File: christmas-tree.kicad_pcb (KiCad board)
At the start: 2 copper layers, 59 x 53 mm, 11 parts, among them IC1 ATTINY85-P, P1 CONN_2, Q1 PHOTO-TRANSISTOR, SW1 SPST

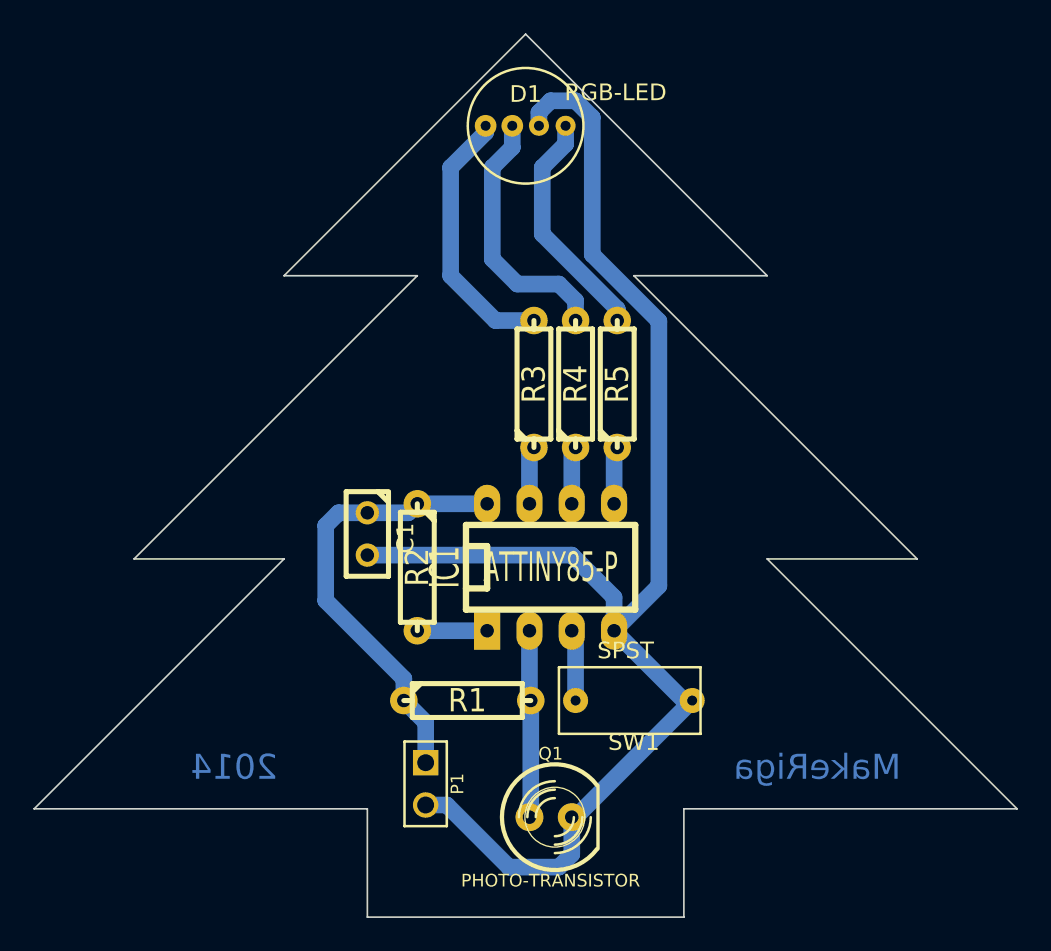
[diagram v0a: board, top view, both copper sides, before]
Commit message: Changes from workstation
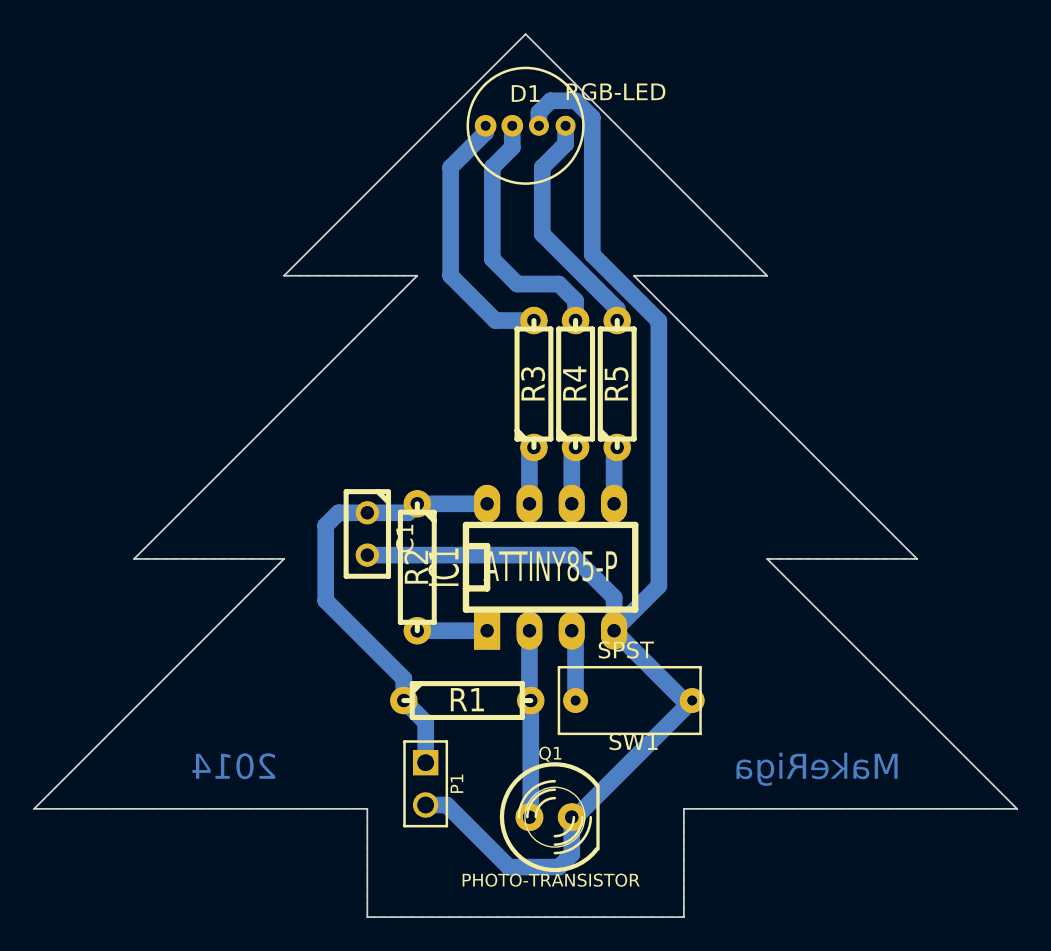
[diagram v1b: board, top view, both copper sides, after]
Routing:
- added copper zone on B.Cu, net (none)
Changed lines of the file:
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@@
     (last_trace_width 1)
     (trace_clearance 0.254)
-    (zone_clearance 0.508)
+    (zone_clearance 1)
     (zone_45_only no)
     (trace_min 0.254)
@@
   (gr_line (start 67 55.5) (end 75 55.5) (angle 90) (layer Edge.Cuts) (width 0.1))
   (gr_line (start 81.5 41) (end 67 55.5) (angle 90) (layer Edge.Cuts) (width 0.1))
-  (segment (start 82.3 46.5) (end 82.3 45.7) (width 1) (layer B.Cu) (net 1) (status 400000))
-  (segment (start 89.5 74.12) (end 86.81 76.81) (width 1) (layer B.Cu) (net 1) (status 800000))
+  (segment (start 82.3 46.5) (end 82.3 45.7) (width 1) (layer B.Cu) (net 1))
+  (segment (start 89.5 74.12) (end 86.81 76.81) (width 1) (layer B.Cu) (net 1))
   (segment (start 89.5 58.226574) (end 89.5 74.12) (width 1) (layer B.Cu) (net 1))
   (segment (start 85.5 54.226574) (end 89.5 58.226574) (width 1) (layer B.Cu) (net 1))
@@
   (segment (start 91.5 81) (end 91 81) (width 1) (layer B.Cu) (net 1))
   (segment (start 91 81) (end 86.81 76.81) (width 1) (layer B.Cu) (net 1))
-  (segment (start 79.1 46.5) (end 79.1 46.9) (width 1) (layer B.Cu) (net 2) (status C00000))
-  (segment (start 79.69 58.19) (end 82 58.19) (width 1) (layer B.Cu) (net 2) (status 800000))
+  (segment (start 79.1 46.5) (end 79.1 46.9) (width 1) (layer B.Cu) (net 2))
+  (segment (start 79.69 58.19) (end 82 58.19) (width 1) (layer B.Cu) (net 2))
   (segment (start 77 55.5) (end 79.69 58.19) (width 1) (layer B.Cu) (net 2))
   (segment (start 77 49) (end 77 55.5) (width 1) (layer B.Cu) (net 2))
-  (segment (start 79.1 46.9) (end 77 49) (width 1) (layer B.Cu) (net 2) (status 400000))
+  (segment (start 79.1 46.9) (end 77 49) (width 1) (layer B.Cu) (net 2))
   (segment (start 86.81 69.19) (end 86.81 66) (width 1) (layer B.Cu) (net 3))
   (segment (start 86.81 66) (end 87 65.81) (width 1) (layer B.Cu) (net 3))
@@
   (segment (start 81.73 76.81) (end 81.73 80.92) (width 1) (layer B.Cu) (net 7))
   (segment (start 81.73 80.92) (end 81.81 81) (width 1) (layer B.Cu) (net 7))
-  (segment (start 87 58.19) (end 87 57.5) (width 1) (layer B.Cu) (net 8) (status C00000))
-  (segment (start 83.9 47.6) (end 83.9 46.5) (width 1) (layer B.Cu) (net 8) (status 800000))
+  (segment (start 87 58.19) (end 87 57.5) (width 1) (layer B.Cu) (net 8))
+  (segment (start 83.9 47.6) (end 83.9 46.5) (width 1) (layer B.Cu) (net 8))
   (segment (start 82.5 49) (end 83.9 47.6) (width 1) (layer B.Cu) (net 8))
   (segment (start 82.5 53) (end 82.5 49) (width 1) (layer B.Cu) (net 8))
-  (segment (start 87 57.5) (end 82.5 53) (width 1) (layer B.Cu) (net 8) (status 400000))
-  (segment (start 80.7 46.5) (end 80.7 47.8) (width 1) (layer B.Cu) (net 9) (status 400000))
-  (segment (start 84.5 57) (end 84.5 58.19) (width 1) (layer B.Cu) (net 9) (status 800000))
+  (segment (start 87 57.5) (end 82.5 53) (width 1) (layer B.Cu) (net 8))
+  (segment (start 80.7 46.5) (end 80.7 47.8) (width 1) (layer B.Cu) (net 9))
+  (segment (start 84.5 57) (end 84.5 58.19) (width 1) (layer B.Cu) (net 9))
   (segment (start 83.5 56) (end 84.5 57) (width 1) (layer B.Cu) (net 9))
   (segment (start 81 56) (end 83.5 56) (width 1) (layer B.Cu) (net 9))
@@
   (segment (start 72 69.73) (end 74.46 69.73) (width 1) (layer B.Cu) (net 11))
   (segment (start 74.46 69.73) (end 75 69.19) (width 1) (layer B.Cu) (net 11))
+  (zone (net 0) (net_name "") (layer B.Cu) (hatch edge 0.508)
+    (connect_pads (clearance 0.2))
+    (min_thickness 0.254)
+    (fill (arc_segments 16) (thermal_gap 0.508) (thermal_bridge_width 0.508))
+    (polygon
+      (pts
+        (xy 111 87.5) (xy 91 87.5) (xy 91 94) (xy 72 94) (xy 72 87.5)
+        (xy 52 87.5) (xy 67 72.5) (xy 58 72.5) (xy 75 55.5) (xy 67 55.5)
+        (xy 81.5 41) (xy 96 55.5) (xy 88 55.5) (xy 105 72.5) (xy 96 72.5)
+        (xy 111 87.5)
+      )
+    )
+  )
 )
